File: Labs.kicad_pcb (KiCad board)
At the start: 2 copper layers, 45.2 x 36.2 mm, 58 parts, among them J1 PROG_port, J2 USB_C_Receptacle_PowerOnly_6P, Q1 AO3401A, SW1BOOT1 SW_Push, SW2NRST1 SW_Push, U1 STM32F407VGTx, U2 TP4056-42-ESOP8, U3 DW01A, U4 8205A, U5 AMS1117-3.3, Y1 Crystal

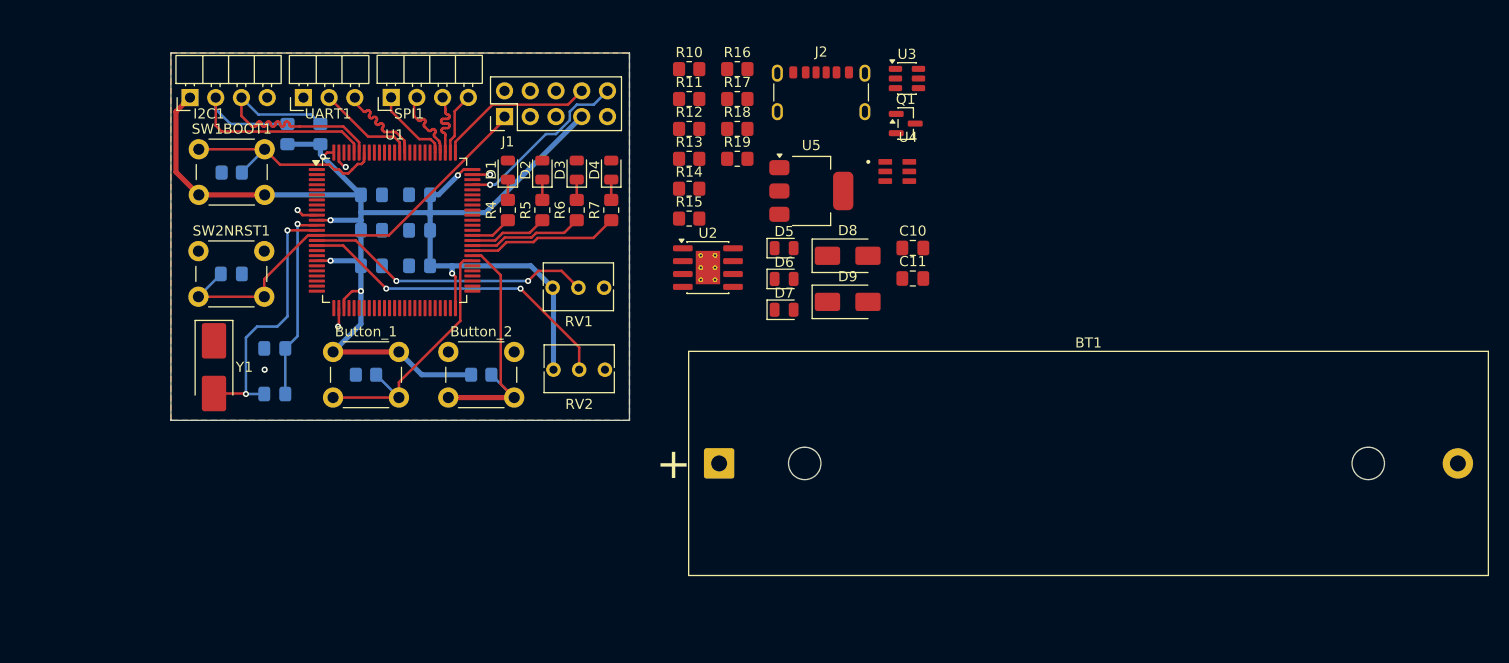
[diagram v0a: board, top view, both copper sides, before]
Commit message: feat: add tracing
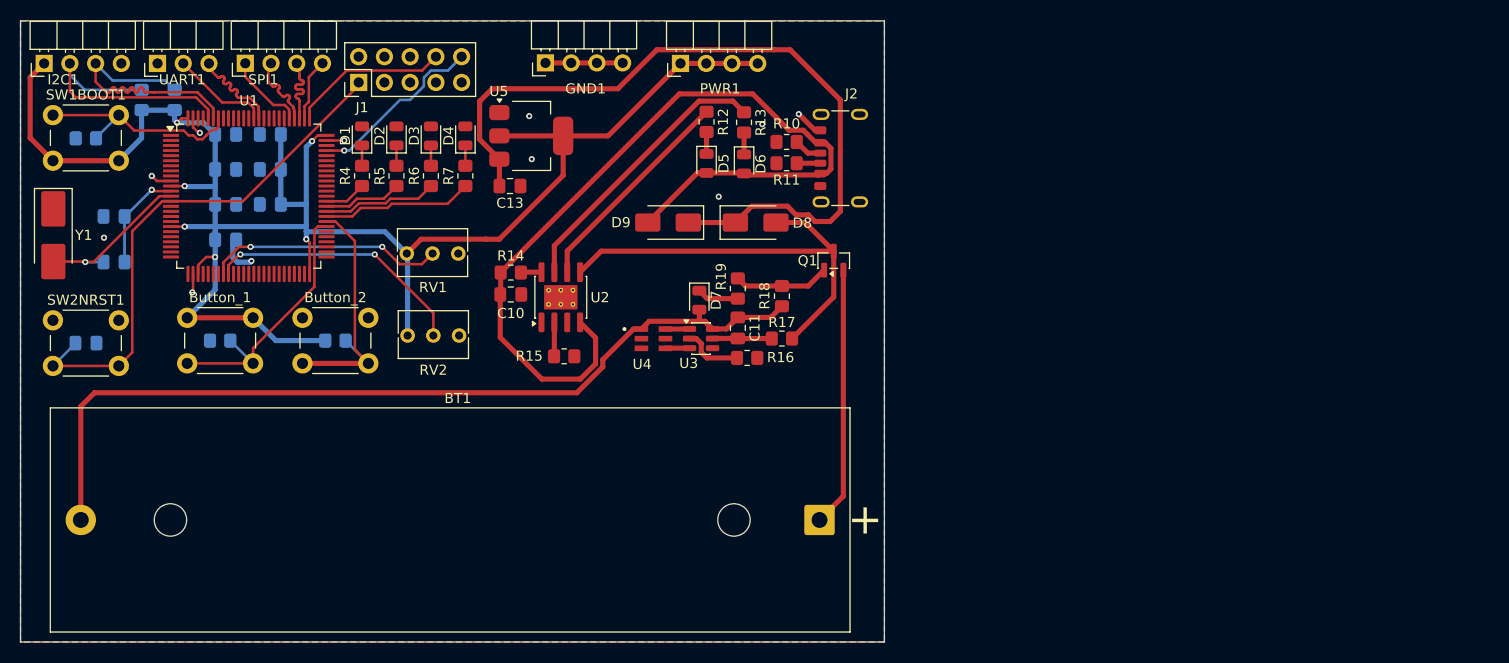
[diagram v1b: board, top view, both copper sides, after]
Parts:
- added C13: C 10 uF, Capacitor_SMD:C_0805_2012Metric_Pad1.18x1.45mm_HandSolder, F.Cu at (158.2, 87.6)
- added C14: C 10 uF, Capacitor_SMD:C_0805_2012Metric_Pad1.18x1.45mm_HandSolder, B.Cu at (134.6, 89.4)
- added GND1: Conn_01x04_Pin, Connector_PinHeader_2.54mm:PinHeader_1x04_P2.54mm_Horizontal, F.Cu at (161.7, 75.5)
- added PWR1: Conn_01x04_Pin, Connector_PinHeader_2.54mm:PinHeader_1x04_P2.54mm_Horizontal, F.Cu at (175.0, 75.5)
- D5: value LED Green -> STANDBY
- D6: value LED Blue -> CHARGE
- D7: value LED Red -> BAT
- moved C10 39.9 mm to (158.3, 98.3)
- moved U3 32.7 mm to (177.1, 102.7)
- moved U4 29.2 mm to (172.4, 102.7)
- moved R16 28.5 mm to (181.6, 104.6), turned to 180 degrees
- moved U5 28.2 mm to (160.3, 82.7)
- moved R17 24.0 mm to (185.0, 102.7), turned to 180 degrees
- moved C2 23.1 mm to (130.2, 82.5), turned to 180 degrees
- moved C3 20.5 mm to (119.1, 90.6)
- moved C5 20.5 mm to (119.1, 95.1)
- moved Y1 20.5 mm to (113.1, 92.5)
- moved C4 20.1 mm to (130.2, 86.0), turned to 180 degrees
- moved R14 19.5 mm to (158.3, 96.2)
- moved D9 19.4 mm to (173.8, 91.2), turned to 180 degrees
- moved C6 19.2 mm to (130.2, 89.4), turned to 180 degrees
- moved R15 18.4 mm to (163.6, 104.4), turned to 180 degrees
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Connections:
- C11 pad 1: Net-(U3-GND) -> Net-(BT1--)
- R17 pad 1: Net-(U2-BAT) -> +BATT
- U1 pad 15: /ADC_1 -> unconnected-(U1-PC0-Pad15)
- U1 pad 16: /ADC_2 -> unconnected-(U1-PC1-Pad16)
- U1 pad 33: unconnected-(U1-PC4-Pad33) -> /ADC_1
- U1 pad 34: unconnected-(U1-PC5-Pad34) -> /ADC_2
- U2 pad 5: Net-(U2-BAT) -> +BATT
- U3 pad 6: Net-(U3-GND) -> Net-(BT1--)
- U4 pad 2: Net-(U4-Pad2) -> unconnected-(U4-Pad2)
- U4 pad 5: Net-(U4-Pad2) -> unconnected-(U4-Pad2)_1
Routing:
- net VBUS: track 0.00 -> 87.4 mm
- net Net-(BT1--): track 0.00 -> 86.7 mm
- net Net-(D8-K): track 0.00 -> 76.7 mm
- net +BATT: track 0.00 -> 43.1 mm
- net +3.3V: track 144.7 -> 183.8 mm
- net Net-(U2-~{CHRG}): track 0.00 -> 27.7 mm
- net Net-(BT1-+): track 0.00 -> 25.6 mm
- net Net-(U2-~{STDBY}): track 0.00 -> 21.5 mm
- net GND: track 7.49 -> 22.9 mm, vias 5 -> 11
- net /EXTAL: track 26.9 -> 16.1 mm, vias 2 -> 1
- net /NRST: track 41.9 -> 52.1 mm
- net Net-(Q1-G): track 0.00 -> 9.52 mm
- net /XTAL: track 19.2 -> 10.2 mm
- net /ADC_2: track 32.3 -> 26.1 mm
- net Net-(U3-CS): track 0.00 -> 5.98 mm
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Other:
- board size 45.2 x 36.2 mm -> 85.2 x 61.3 mm
